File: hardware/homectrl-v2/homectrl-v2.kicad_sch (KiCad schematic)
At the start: 57 parts, among them J1 Barrel_Jack, Q1 DMP6023LE-13, Q2 2N7002, U1 TPS5405DR, U2 AMS1117-3.3, U3 DMP4065S-7, U4 ESP32-S3-WROOM-1

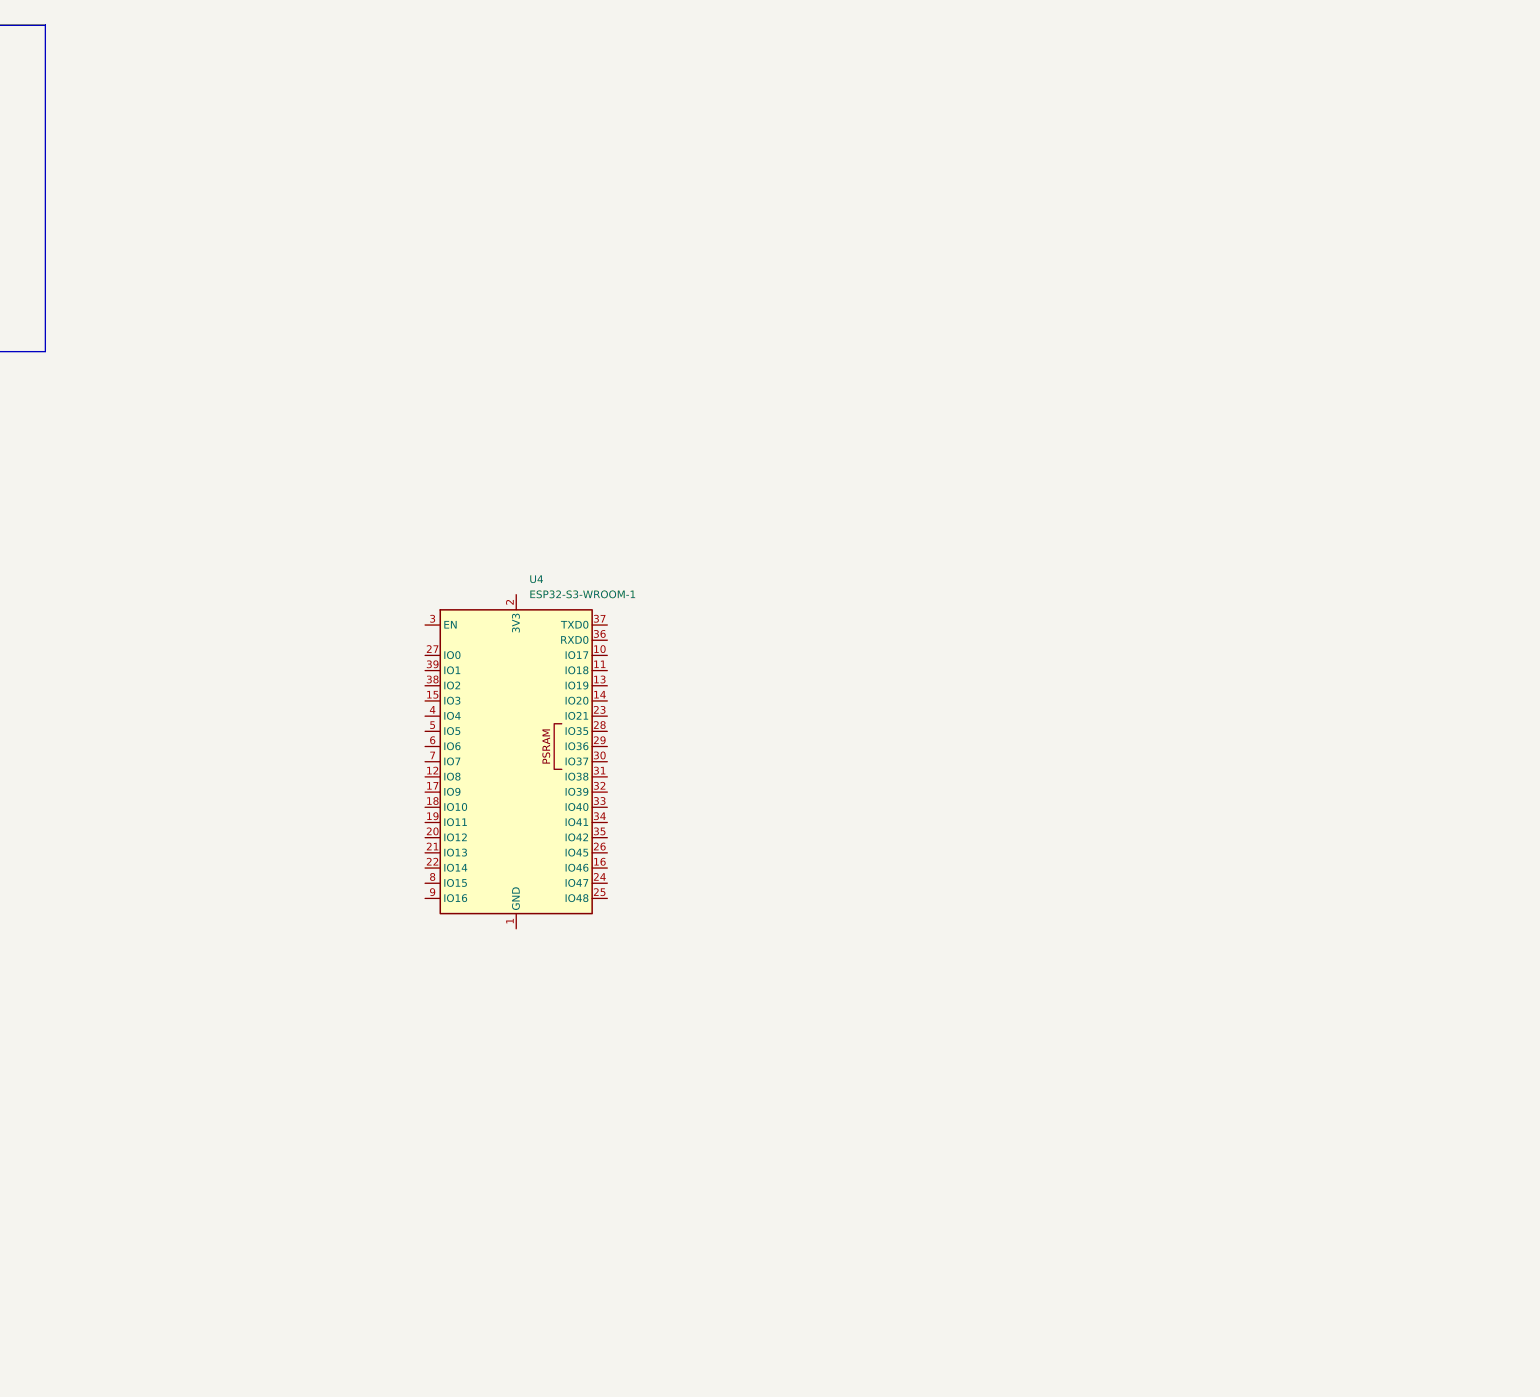
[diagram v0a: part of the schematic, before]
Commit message: sch work
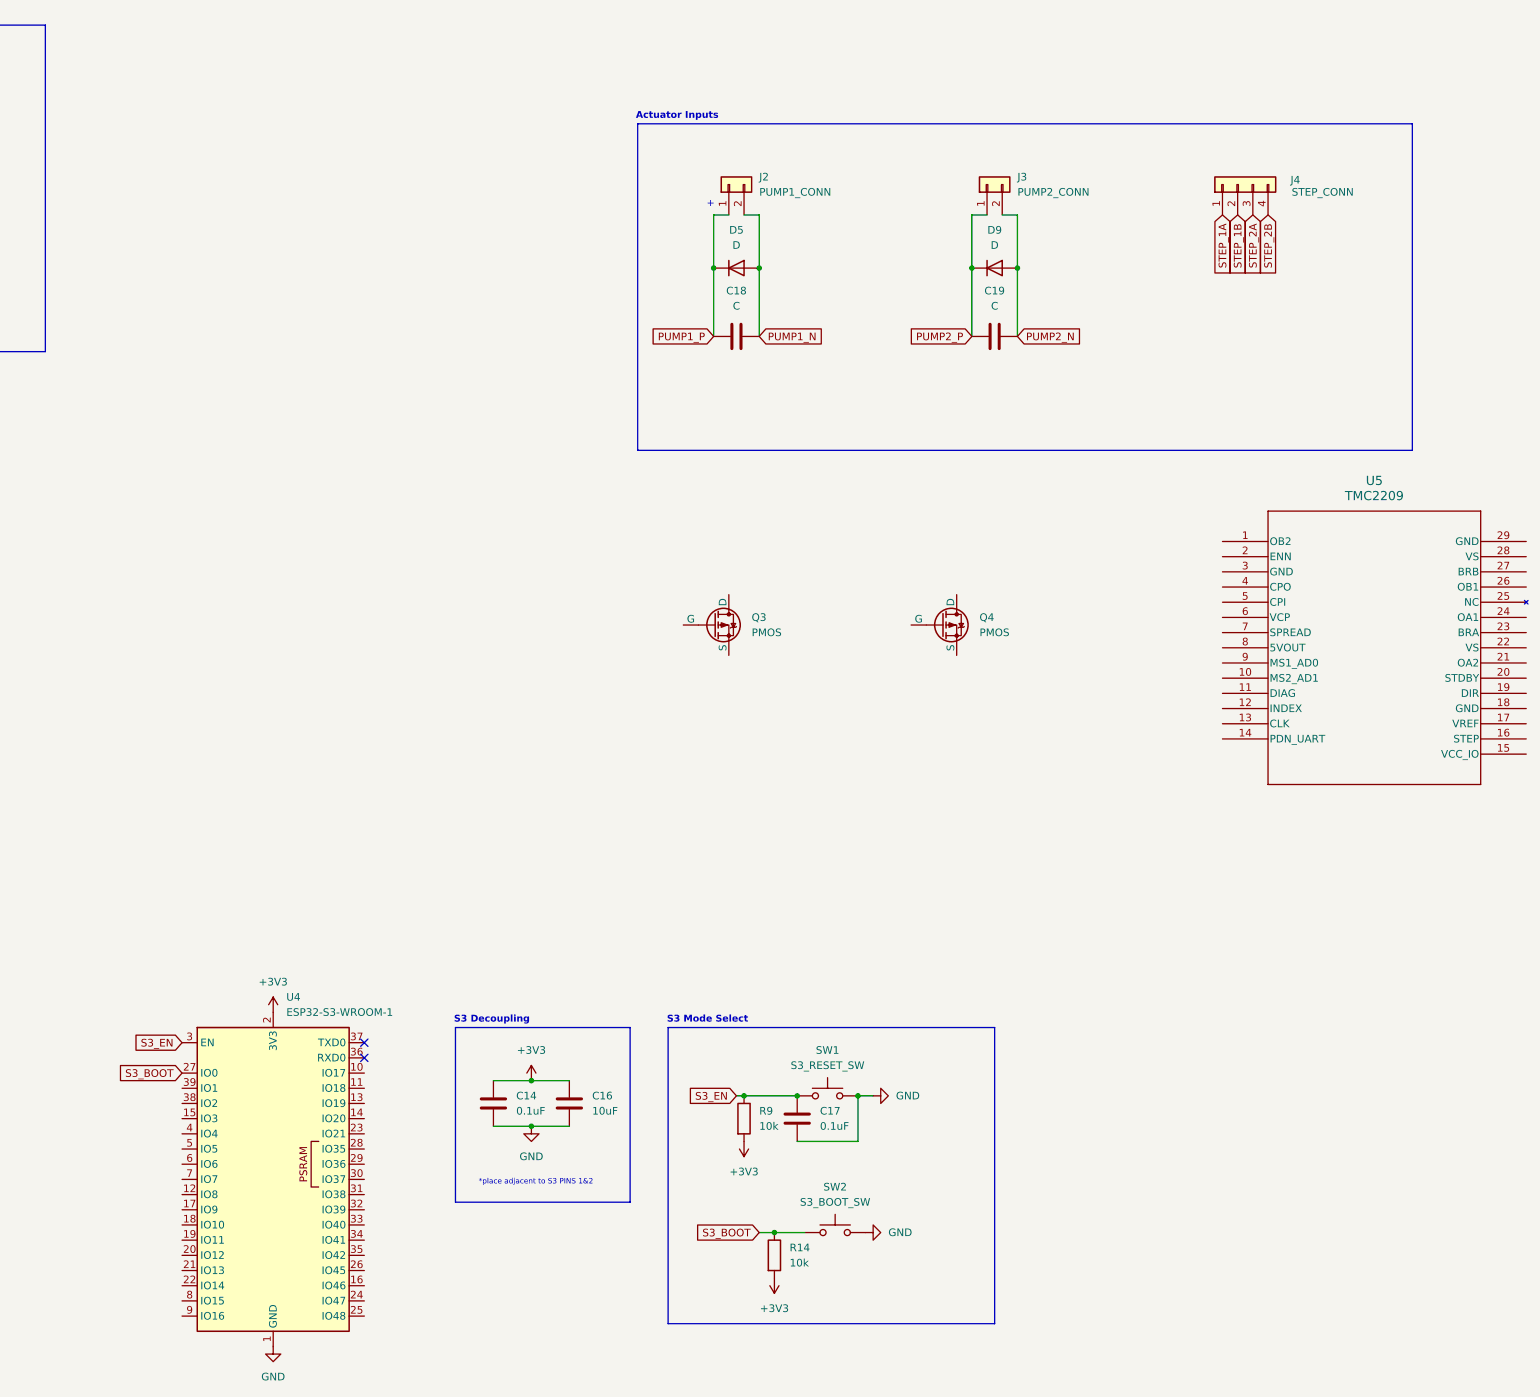
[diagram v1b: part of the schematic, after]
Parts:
- added C14, C17: 0.1uF, Capacitor_SMD:C_0402_1005Metric, symbol Device:C
- added C16: 10uF, Capacitor_SMD:C_0603_1608Metric, symbol Device:C
- added C18, C19: C, symbol Device:C
- added D5, D9: D, symbol Device:D
- added J2: PUMP1_CONN, symbol Connector_Generic:Conn_01x02
- added J3: PUMP2_CONN, symbol Connector_Generic:Conn_01x02
- added J4: STEP_CONN, symbol Connector_Generic:Conn_01x04
- added Q3, Q4: PMOS, symbol Simulation_SPICE:PMOS
- added R14, R9: 10k, Resistor_SMD:R_0402_1005Metric, symbol Device:R
- added SW1: S3_RESET_SW, symbol Switch:SW_Push
- added SW2: S3_BOOT_SW, symbol Switch:SW_Push
- added U5: TMC2209, QFN28_5X5_TRI, symbol TMC2209:TMC2209
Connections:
- net +3V3: now also U4.2 (3V3), C14.1, C16.1, R14.2, R9.2
- net GND: now also U4.1 (GND), U4.40 (GND), U4.41 (GND), C14.2, C16.2, C17.2, SW1.2, SW2.2
- net S3_BOOT: now reaches U4.27 (IO0)
- net S3_BOOT: now also R14.1, SW2.1
- net S3_EN: now reaches U4.3 (EN)
- net S3_EN: now also C17.1, R9.1, SW1.1
- new net PUMP1_N: C18.2, D5.2 (A), J2.2 (Pin_2)
- new net PUMP1_P: C18.1, D5.1 (K), J2.1 (Pin_1)
- new net PUMP2_N: C19.2, D9.2 (A), J3.2 (Pin_2)
- new net PUMP2_P: C19.1, D9.1 (K), J3.1 (Pin_1)
- new net STEP_1A: J4.1 (Pin_1)
- new net STEP_1B: J4.2 (Pin_2)
- new net STEP_2A: J4.3 (Pin_3)
- new net STEP_2B: J4.4 (Pin_4)
- no-connect marks 0 -> 2
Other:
- note added: "*place adjacent to S3 PINS 1&2"
- note added: "+"
- note added: "Actuator Inputs"
- note added: "S3 Decoupling"
- note added: "S3 Mode Select"
- moved on the sheet: U4

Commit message: entry circuits
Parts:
- added BZ1: SMT-0540-S-R, SMT-0540-S-R:XDCR_SMT-0540-S-R, symbol SMT-0540-S-R:SMT-0540-S-R
- added C20, C21: 0.1uF, Capacitor_SMD:C_0402_1005Metric, symbol Device:C
- added D11: WIFI_LED, LED_SMD:LED_0603_1608Metric, symbol Device:LED
- added D12: DBG_LED, LED_SMD:LED_0603_1608Metric, symbol Device:LED
- added D13: 1N4148W, Diode_SMD:D_SOD-123, symbol Device:D
- added D14: SYS_LED, LED_SMD:LED_WS2812B-Mini_PLCC4_3.5x3.5mm, symbol LED:WS2812B
- added J5: USB_C_CONN, Connector_USB:USB_C_Receptacle_G-Switch_GT-USB-7010ASV, symbol USB_C:USB_C_Female_USB2_Small
- added J6: SMS1_CONN, symbol Connector_Generic:Conn_01x04
- added J7: SMS2_CONN, symbol Connector_Generic:Conn_01x04
- added J8: FSW1_CONN, symbol Connector_Generic:Conn_01x02
- added J9: FSW2_CONN, symbol Connector_Generic:Conn_01x02
- added Q5: AO3400A, Package_TO_SOT_SMD:SOT-23, symbol Transistor_FET:2N7002
- added R16: 200, Resistor_SMD:R_0402_1005Metric, symbol Device:R
- added R17: 330, Resistor_SMD:R_0402_1005Metric, symbol Device:R
- added R18: 150, Resistor_SMD:R_0402_1005Metric, symbol Device:R
- added R19: 10k, Resistor_SMD:R_0402_1005Metric, symbol Device:R
- added R20, R21: 5.1k, Resistor_SMD:R_0603_1608Metric, symbol Device:R
- added U6: ADS1115IDGS, Package_SO:TSSOP-10_3x3mm_P0.5mm, symbol Analog_ADC:ADS1115IDGS
- added U8, U9: TPD2E001DRLR, TPD2E001DRLR:SOT50P160X60-5N, symbol TPD2E001DRLR:TPD2E001DRLR
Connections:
- net +3V3: now also BZ1.LEAD+, C20.1, C21.1, D13.1 (K), D14.1 (VDD)
- net 5V_USB: now also J5.A4 (VBUS), J5.A9 (VBUS), J5.B4 (VBUS), J5.B9 (VBUS)
- net GND: now also C20.2, C21.2, D11.1 (K), D12.1 (K), D14.3 (VSS), J5.A1 (GND), J5.A12 (GND), J5.B1 (GND), J5.B12 (GND), J5.S1 (SHIELD), Q5.2 (S), R19.1, R20.2, R21.2
- new net: Q5.1 (G), R16.1, R19.2
- new net: BZ1.LEAD-, D13.2 (A), Q5.3 (D)
- new net: J5.B5 (CC2), R21.1
- new net: J5.A5 (CC1), R20.1
- new net: D11.2 (A), R17.2
- new net: D12.2 (A), R18.2
- new net BUZZ_EN: R16.2
- new net DBG_LED: R17.1
- new net RGB_DATA: D14.4 (DIN)
- new net USB_N: J5.A7 (D-), J5.B7 (D-)
- new net USB_P: J5.A6 (D+), J5.B6 (D+)
- new net WIFI_LED: R18.1
- no-connect marks 2 -> 5
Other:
- note added: "Analog Digital Conversion"
- note added: "Buzzer Driver"
- note added: "LED Diagnosis & Indication"
- note added: "Sensor Inputs"
- note added: "Switch Inputs"
- note added: "USB Connector"
- note added: "Vf = 2.1V, R = 68, If = 0.02A * 150 selected for dimness"
- note added: "Vf = 2.8V, R = 100, If = 0.005A * 330 selected for dimness"
- note added: "flyback diode to protect against inductive spikes"
- company: (none) -> Jeevan Sanchez
- title: (none) -> homectrl V2
- moved on the sheet: C18, C19, D5, D9, J2, J3, J4, Q3, Q4, U5
